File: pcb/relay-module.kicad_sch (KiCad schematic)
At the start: 57 parts, among them J1 AVR-UPDI-6, J2 QWICC, J3 Power In, J4 Power Out, K1 PR24-5V-900-1A, P1 MountingHole_Pad, P2 MountingHole_Pad, P3 MountingHole_Pad, P4 MountingHole_Pad, Q1 MMBT3904, U1 ATtiny1616-MNR, U3 LTV-356T

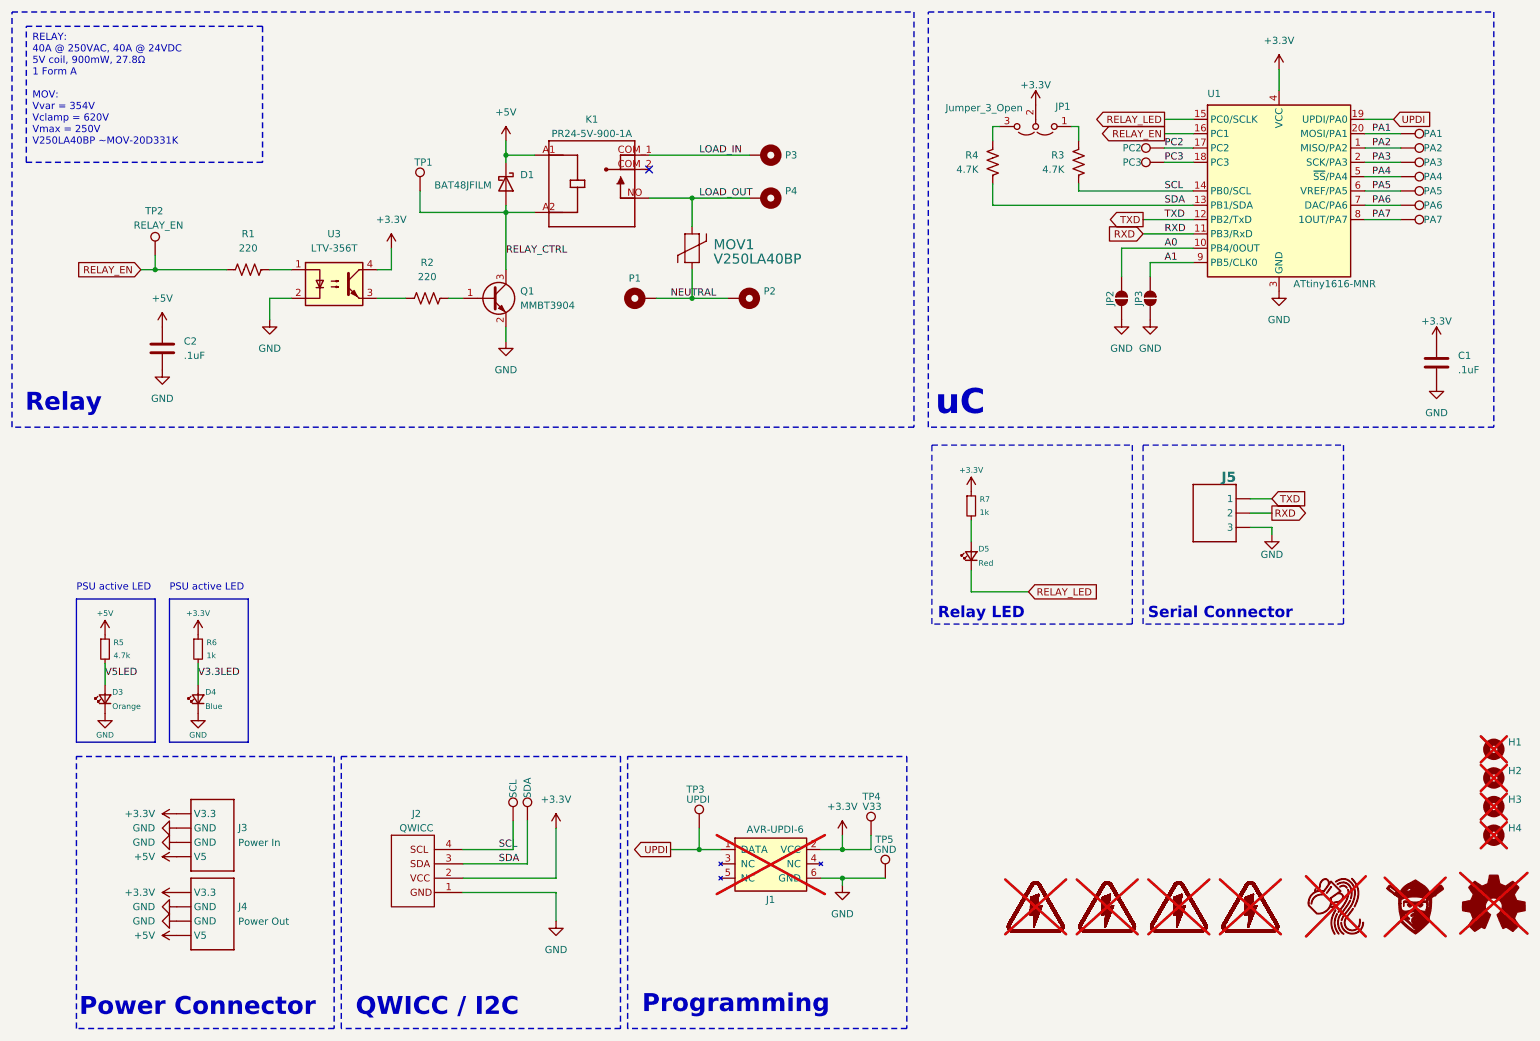
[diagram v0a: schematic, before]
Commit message: schematic and PCB clean up
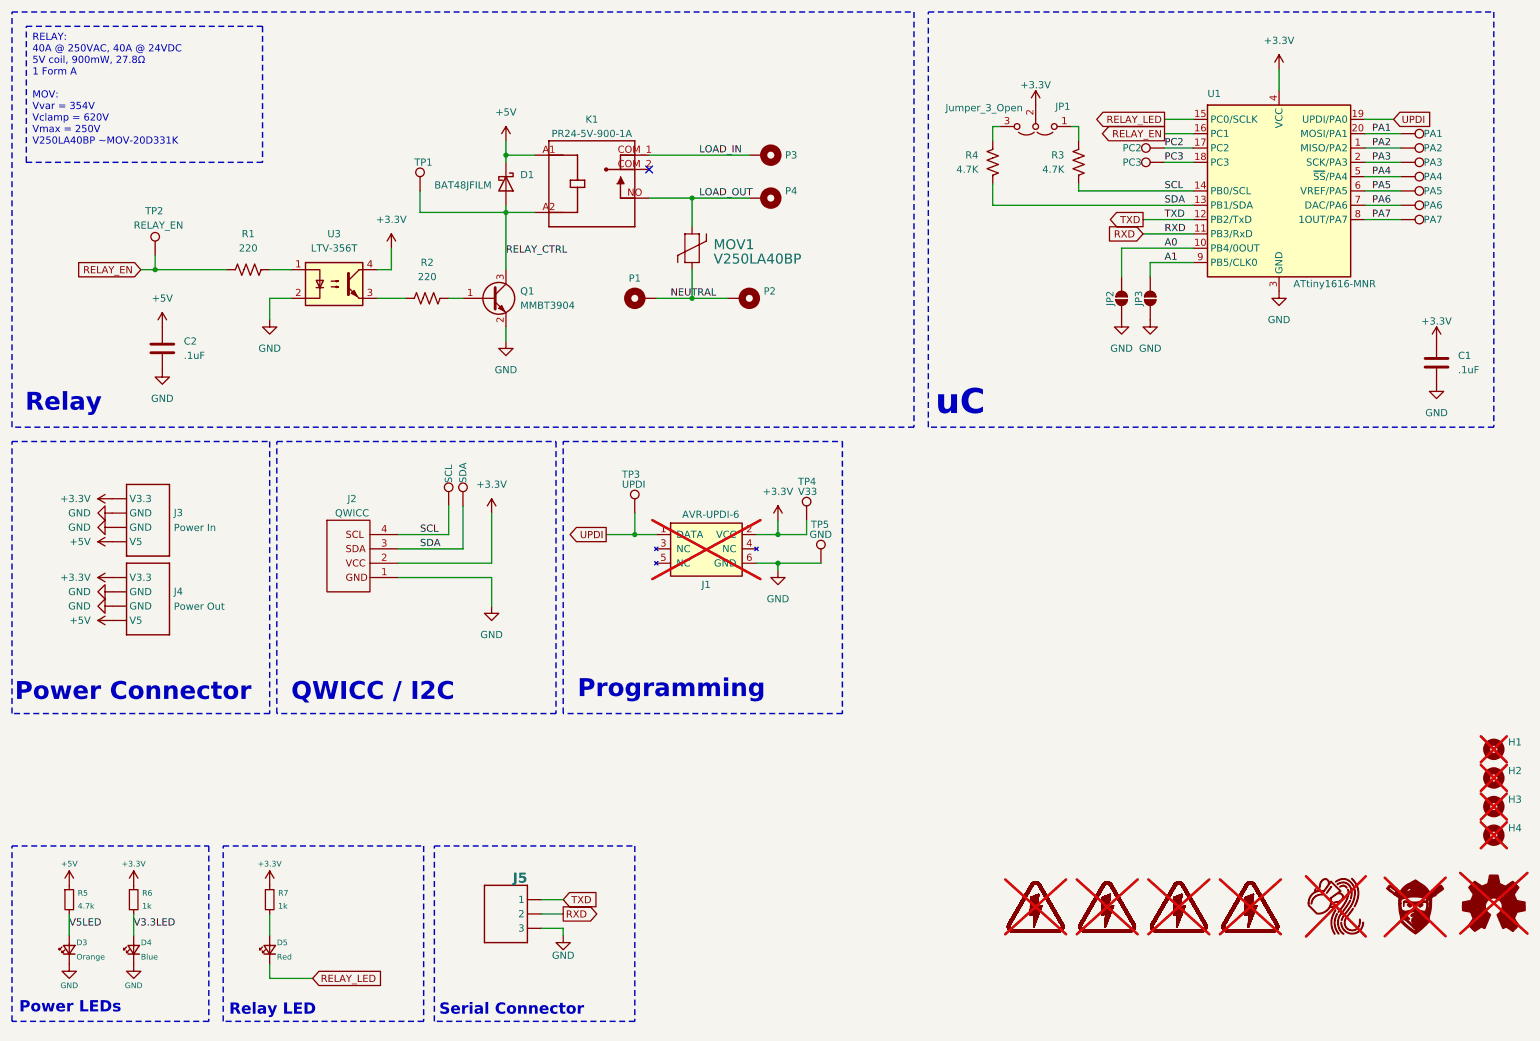
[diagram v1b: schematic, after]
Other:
- note added: "Power LEDs"
- note removed: "PSU active LED"
- moved on the sheet: D3, D4, D5, J1, J2, J3, J4, J5, R5, R6, R7, TP3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
